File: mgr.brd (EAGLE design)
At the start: 100 x 80 mm, 41 parts, among them CN1 USB, CN2 SWD, CN3 BT, CN4 SF-MICROSD, IC1 LM2936DT-3.3, U2 LSM9DS0, U3 MPL115A, X1 16MHz, X2 32.768kHz

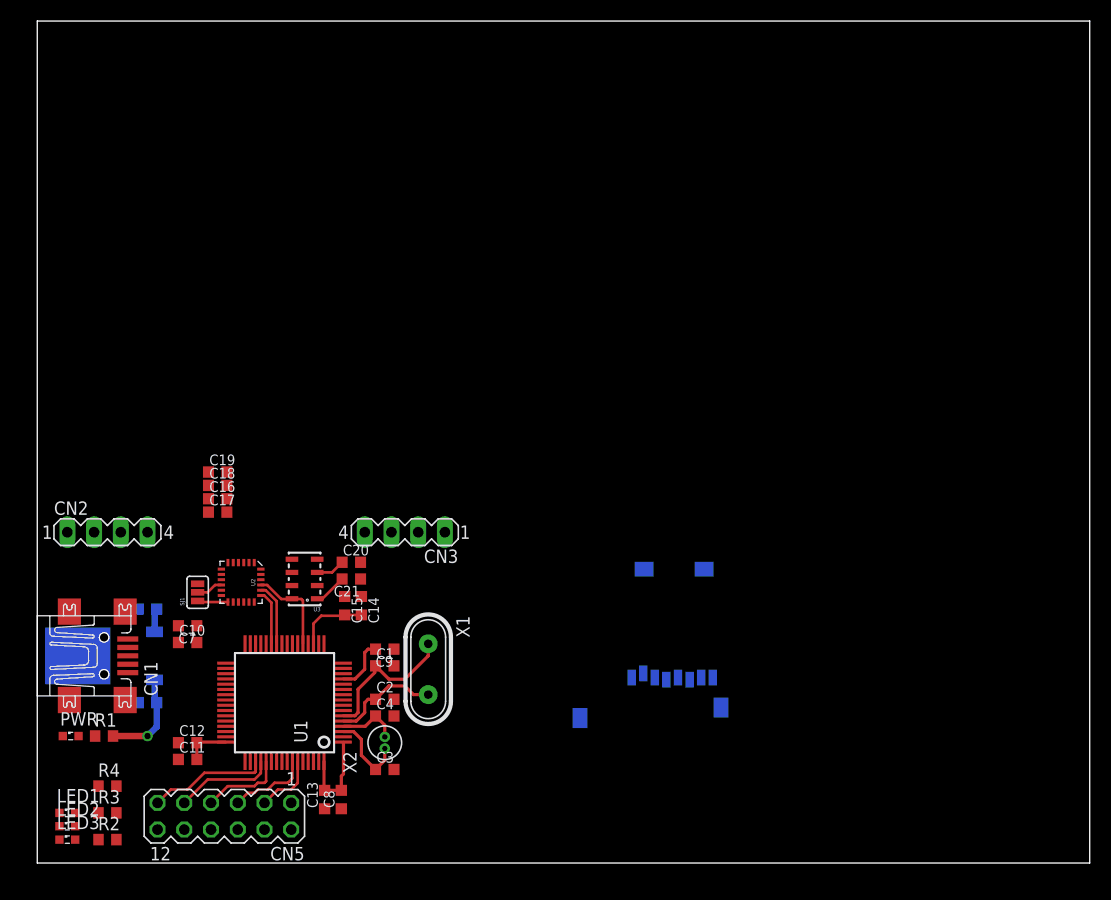
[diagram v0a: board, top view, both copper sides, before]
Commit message: initial commit
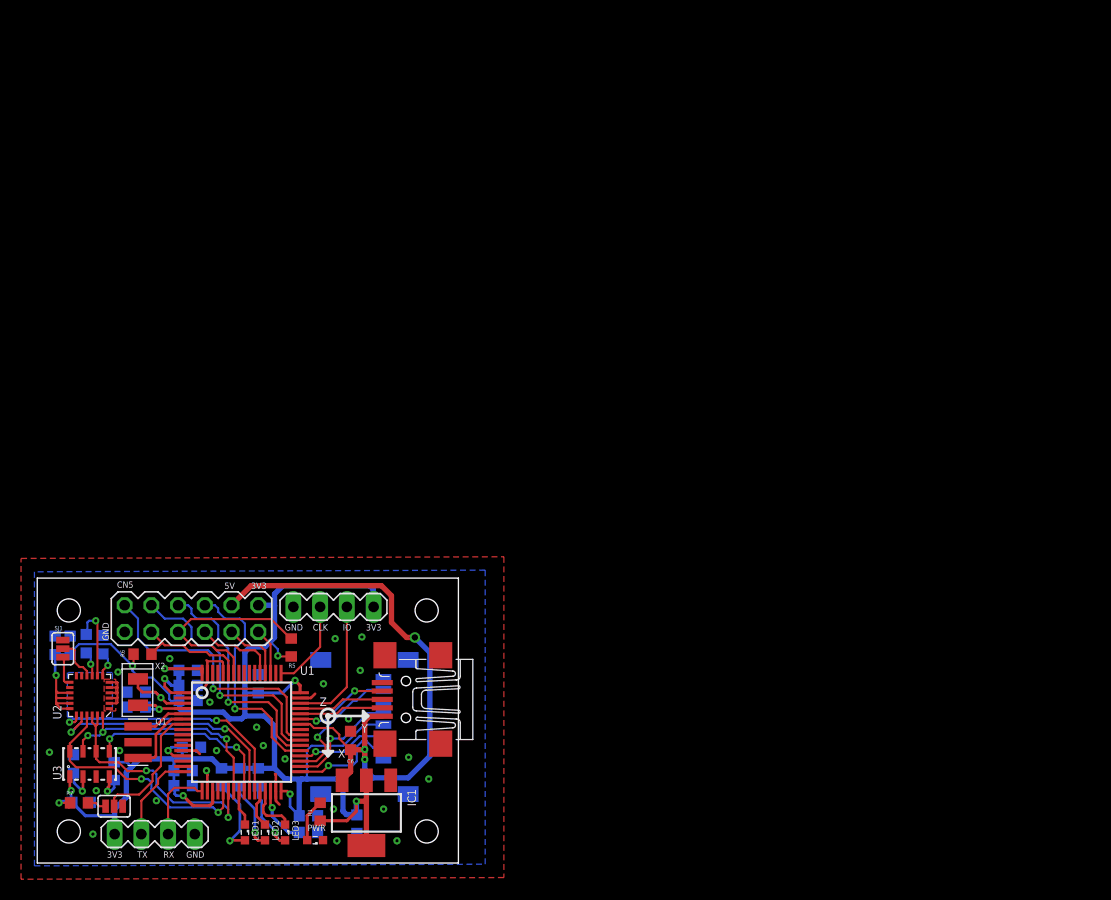
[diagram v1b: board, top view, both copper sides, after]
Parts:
- removed C1, C2: (no value), resistor:C0603K
- removed X1: 16MHz, IQD-Frequency-Products:HC49
- added Q1: 8MHz, murata-filter:CSTCR6M
- added R5, R6: 4k7, resistor:R0603
- added R7, R8: 100k, resistor:R0603
- added SJ2: RESET, SparkFun-Passives:PAD-JUMPER-3-NO_YES_SILK
- CN3: value BT -> UART
- CN4: value SF-MICROSD -> MICRO_SD_CONNECTOR; device microsd:MICROSD -> mgr_con_sd:MICROSD_CONNECTOR
- IC1: value LM2936DT-3.3 -> LM1117IMPX-3.3; device national-semiconductor:TO252 -> lm1117:SOT223
- SJ1: value JUMPER-PAD-3-NOYES_SILK -> (none)
- X2: device IQD-Frequency-Products:WATCH-3X8 -> IQD-Frequency-Products:3.2X1.5-2-PAD
- moved CN3 37.3 mm to (11.2, 2.75), turned to 0 degrees
- moved C21 33.3 mm to (4.17, 5.76), flipped to the bottom, turned to 0 degrees
- moved C20 32.6 mm to (3.44, 9.41), flipped to the bottom, turned to 270 degrees
- moved CN4 30.8 mm to (28.6, 12.4), turned to 270 degrees
- moved IC1 29.0 mm to (31.3, 4.76), flipped to the top, turned to 180 degrees
- moved CN1 29.0 mm to (35.0, 15.5), turned to 180 degrees
- moved U3 26.9 mm to (4.97, 9.41), turned to 90 degrees
- moved PWR 25.2 mm to (26.4, 2.17), turned to 180 degrees
- moved C3 24.7 mm to (9.41, 16.2), flipped to the bottom
- moved C14 24.1 mm to (13.9, 7.35), flipped to the bottom, turned to 0 degrees
- moved X2 23.9 mm to (9.57, 16.2), turned to 270 degrees
- moved C4 23.6 mm to (9.41, 14.8), flipped to the bottom
- moved C5 23.0 mm to (30.4, 3.70), turned to 90 degrees
- moved C6 23.0 mm to (29.8, 11.6), flipped to the top, turned to 270 degrees
- moved C7 22.7 mm to (25.8, 2.90), flipped to the bottom
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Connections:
- removed net BOOT0: U1.60
- removed net PA9: U1.42
- removed net PB10: U1.29
- removed net PB2: U1.28
- new net N$11: R7.2, SJ2.1
- net +3V3: now also IC1.TAB, R2.2, R3.2, R4.2, R5.1, R6.1, R7.1, R8.1; no longer LED1.C, LED2.C, LED3.C
- net +5V: now also IC1.3, U1.42; no longer IC1.1
- net GND: now also IC1.1, Q1.2, SJ2.3, U1.60; no longer C1.2, C2.2, IC1.3
- net LED1: now also LED1.C, U1.24; no longer R2.1
- net LED2: now also LED2.C, U1.28; no longer R3.1
- net LED3: now also LED3.C, U1.29; no longer R4.1
- net N$5: now also R2.1; no longer R2.2
- net N$6: now also R3.1; no longer R3.2
- net N$7: now also R4.1; no longer R4.2
- net NRST: now also SJ2.2
- net OSC_IN: now also Q1.1; no longer C2.1, X1.2
- net OSC_OUT: now also Q1.3; no longer C1.1, X1.1
- net PB6: now also R5.2
- net PB7: now also R6.2
- net SHDN: now also R8.2; no longer U1.24
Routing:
- net +3V3: track 37.5 -> 181.4 mm, vias 1 -> 12
- net +5V: track 2.25 -> 59.0 mm, vias 0 -> 3
- net PC9: track 0.00 -> 26.7 mm, vias 0 -> 1
- net PC8: track 0.00 -> 24.1 mm, vias 0 -> 1
- net MISO1: track 0.01 -> 23.9 mm, vias 0 -> 2
- net PC7: track 0.00 -> 22.5 mm, vias 0 -> 1
- net MOSI1: track 0.00 -> 22.4 mm, vias 0 -> 3
- net PC6: track 0.00 -> 22.1 mm, vias 0 -> 1
- net CS_G: track 5.19 -> 24.2 mm, vias 0 -> 2
- net CS_XM: track 5.97 -> 24.7 mm, vias 0 -> 2
- net CS_MLP: track 0.00 -> 18.5 mm, vias 0 -> 2
- net GND: track 2.77 -> 19.4 mm, vias 0 -> 24
- net SCK1: track 8.73 -> 23.7 mm, vias 0 -> 2
- net SWDIO: track 0.00 -> 12.7 mm
- net MISO2: track 0.00 -> 12.6 mm, vias 0 -> 1
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- added copper zone on layer 1, net GND
- added copper zone on layer 16, net GND
- added copper zone on layer 16, net N$12
- added copper zone on layer 1, net N$9
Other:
- board size 100 x 80 mm -> 40 x 27.1 mm
- board text added: "3V3"
- board text added: "5V"
- board text added: "CLK"
- board text added: "GND"
- board text added: "IO"
- board text added: "RX"
- board text added: "TX"
- board text added: "X"
- board text added: "Y"
- board text added: "Z"
- board text added: "wiktor.sienkiewicz@gmail.com"
